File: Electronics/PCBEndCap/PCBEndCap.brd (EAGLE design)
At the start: 62.9 x 31.1 mm, 2 parts, among them J3 CONNECTOR_9PIN, J4 CONNECTOR_9PIN

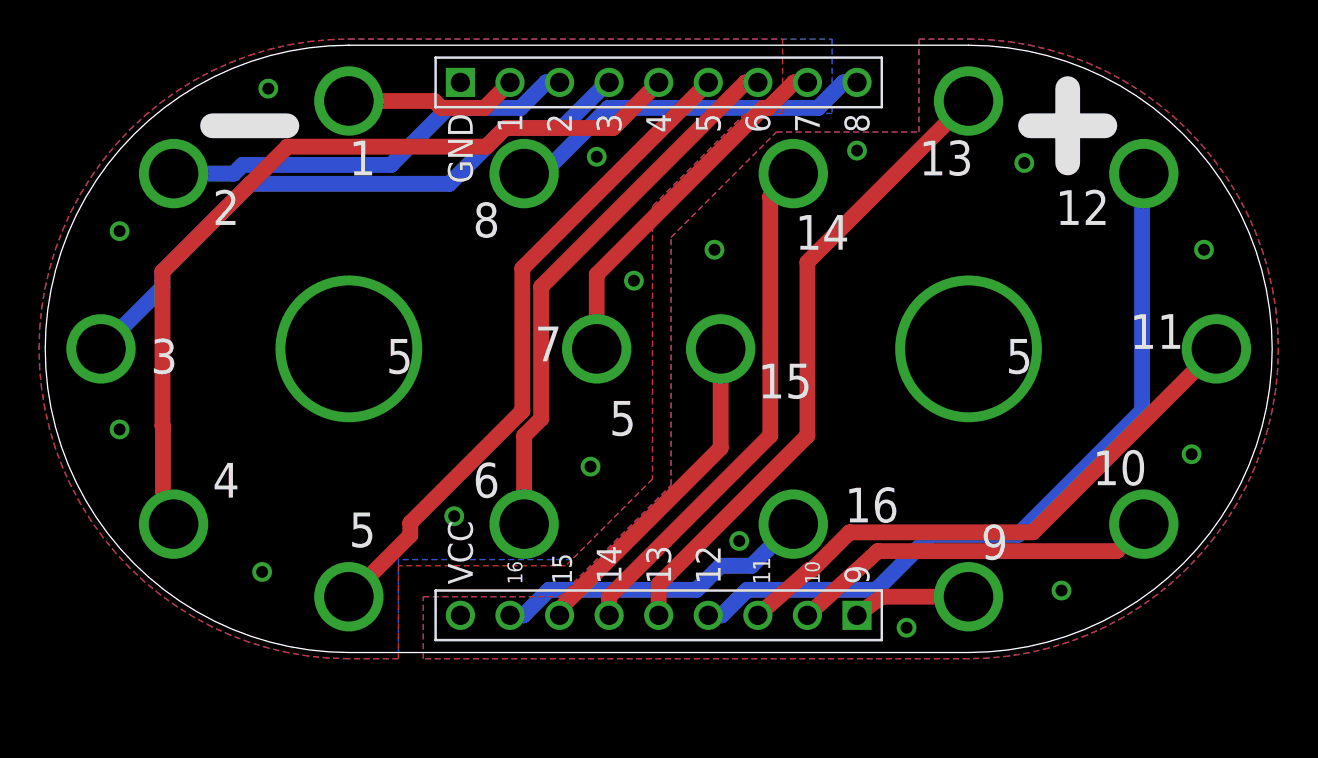
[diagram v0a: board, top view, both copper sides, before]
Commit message: pcb spacer and breakoutoard over
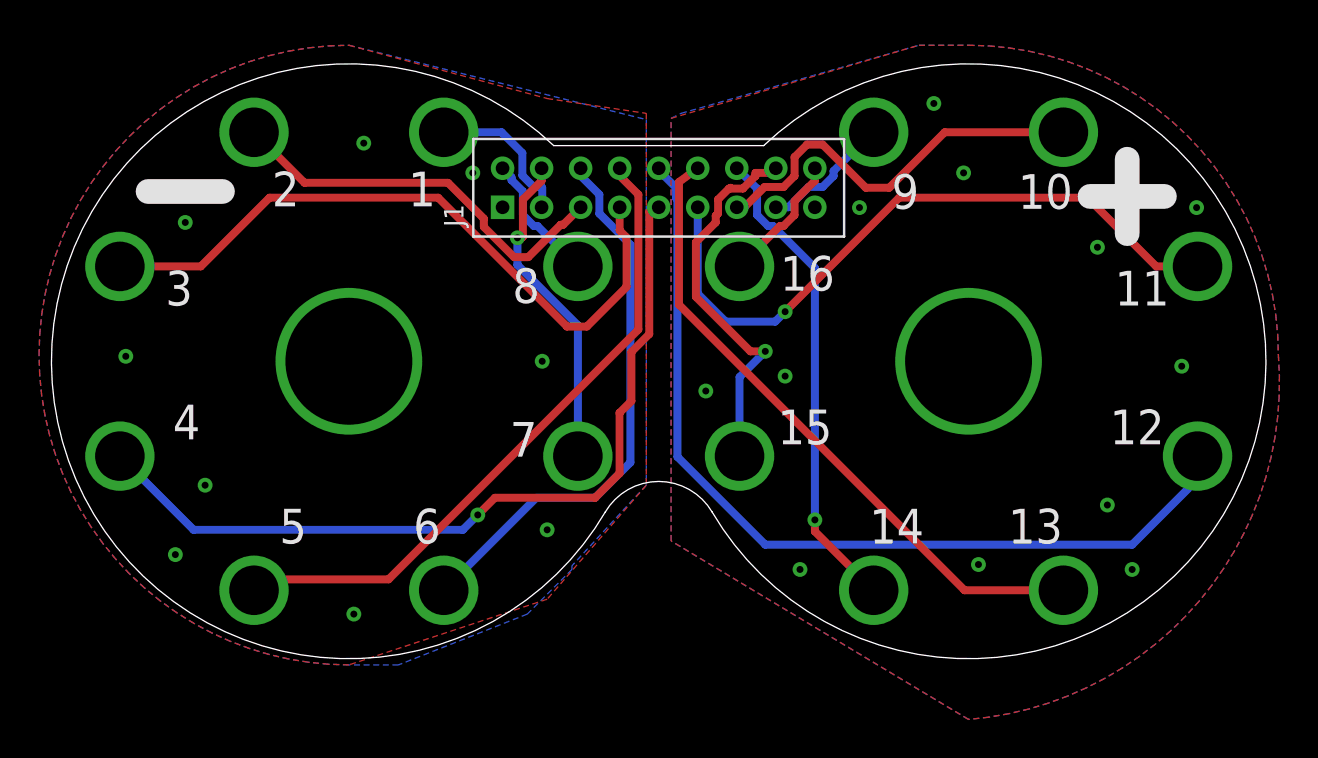
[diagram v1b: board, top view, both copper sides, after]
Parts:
- removed J3, J4: CONNECTOR_9PIN, lolomolo:9PIN_.1'
- added J1: CONNECTORJST2X9_2MM, MarkIIEaglelbr:CONNECTOR9X2_2MMPITCH
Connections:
- removed net N1: J3.2
- removed net N10: J4.2
- removed net N11: J4.3
- removed net N12: J4.4
- removed net N13: J4.5
- removed net N14: J4.6
- removed net N15: J4.7
- removed net N16: J4.8
- removed net N2: J3.3
- removed net N3: J3.4
- removed net N4: J3.5
- removed net N5: J3.6
- removed net N6: J3.7
- removed net N7: J3.8
- removed net N8: J3.9
- removed net N9: J4.1
- new net B1: J1.P$2
- new net B10: J1.P$7
- new net B11: J1.P$6
- new net B12: J1.P$14
- new net B13: J1.P$13
- new net B14: J1.P$12
- new net B15: J1.P$11
- new net B16: J1.P$10
- new net B2: J1.P$3
- new net B3: J1.P$4
- new net B4: J1.P$5
- new net B5: J1.P$15
- new net B6: J1.P$16
- new net B7: J1.P$17
- new net B8: J1.P$18
- new net B9: J1.P$8
- net GND: now also J1.P$1; no longer J3.1
- net VCC: now also J1.P$9; no longer J4.9
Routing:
- net B12: track 0.00 -> 46.3 mm, vias 0 -> 1
- net B4: track 0.00 -> 42.9 mm, vias 0 -> 2
- net N4: track 42.6 -> 0.00 mm, vias 1 -> 0
- net N12: track 38.8 -> 0.00 mm, vias 1 -> 0
- net B3: track 0.00 -> 35.4 mm, vias 0 -> 1
- net B11: track 0.00 -> 34.7 mm, vias 0 -> 2
- net N5: track 34.0 -> 0.00 mm, vias 1 -> 0
- net B5: track 0.00 -> 33.9 mm, vias 0 -> 1
- net B13: track 0.00 -> 33.2 mm, vias 0 -> 1
- net N13: track 32.9 -> 0.00 mm, vias 1 -> 0
- net N3: track 32.2 -> 0.00 mm, vias 1 -> 0
- net N11: track 29.1 -> 0.00 mm, vias 1 -> 0
- net B6: track 0.00 -> 28.4 mm, vias 0 -> 1
- net N6: track 28.0 -> 0.00 mm, vias 1 -> 0
- net N14: track 26.5 -> 0.00 mm, vias 1 -> 0
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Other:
- board size 62.9 x 31.1 mm -> 62.2 x 30.5 mm
- board text removed: "GND"
- board text removed: "VCC"
